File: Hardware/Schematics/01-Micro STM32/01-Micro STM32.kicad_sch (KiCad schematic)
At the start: 0 parts

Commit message: update
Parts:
- added J1: Screw_Terminal_01x04, symbol Connector:Screw_Terminal_01x04
- added U1: MCP23017_ML, Package_DFN_QFN:QFN-28-1EP_6x6mm_P0.65mm_EP4.25x4.25mm, symbol Interface_Expansion:MCP23017_ML
- added U2: ESP32-DEVKITC-32D, ESP32-DEVKITC-32D:MODULE_ESP32-DEVKITC-32D, symbol ESP32-DEVKITC-32D:ESP32-DEVKITC-32D
- added U3, U4: 74HCT138, symbol 74xx:74HCT138
- added U69A: AD8604ARUZ, AD8604ARUZ:SOP65P640X120-14N, symbol AD8604ARUZ:AD8604ARUZ

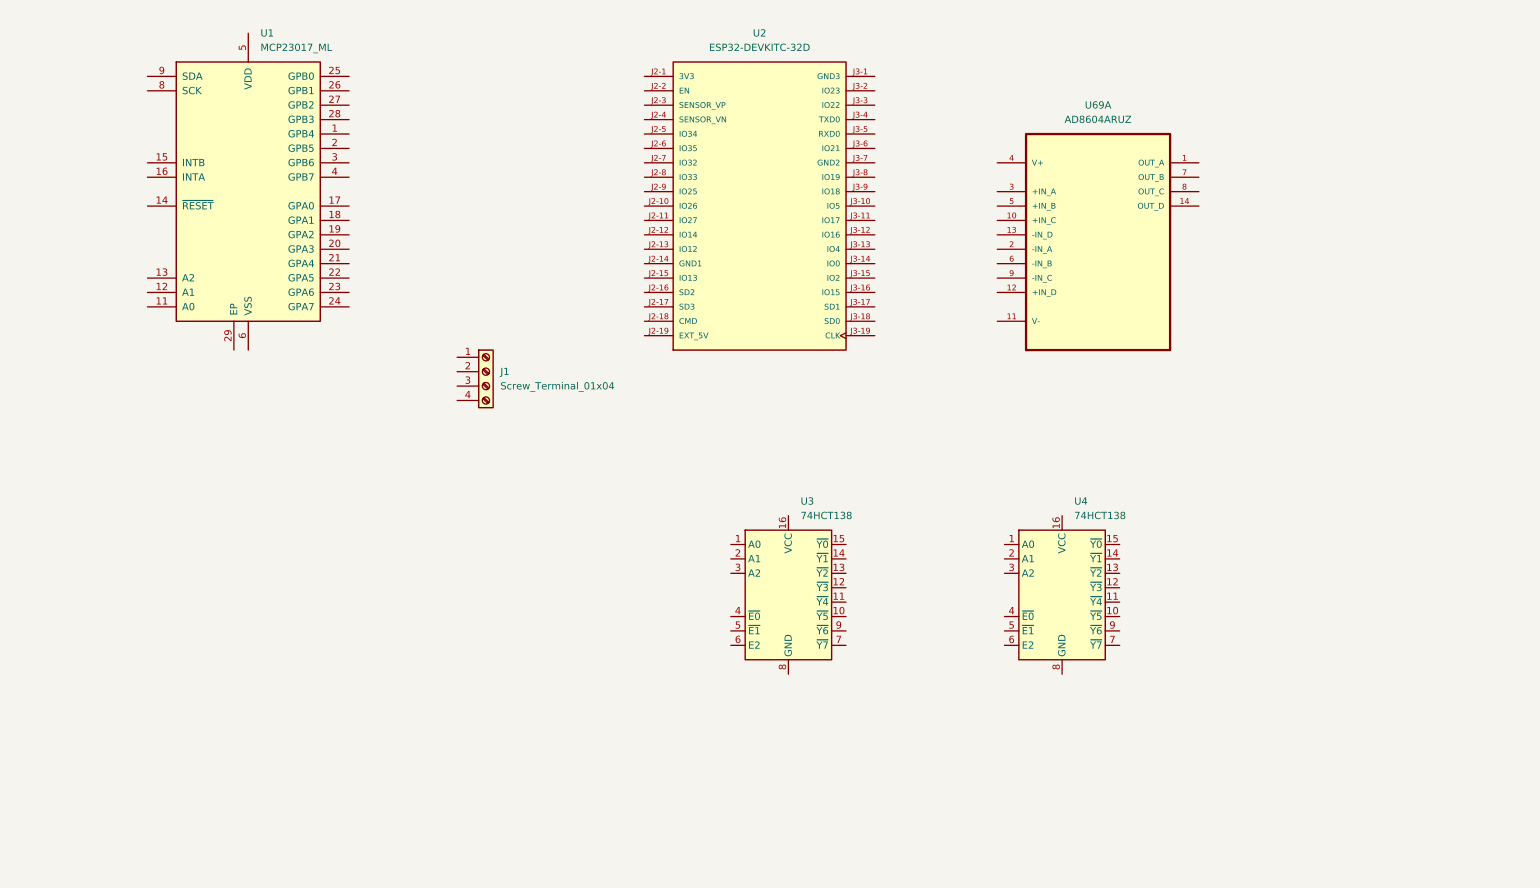
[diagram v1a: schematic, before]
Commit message: update
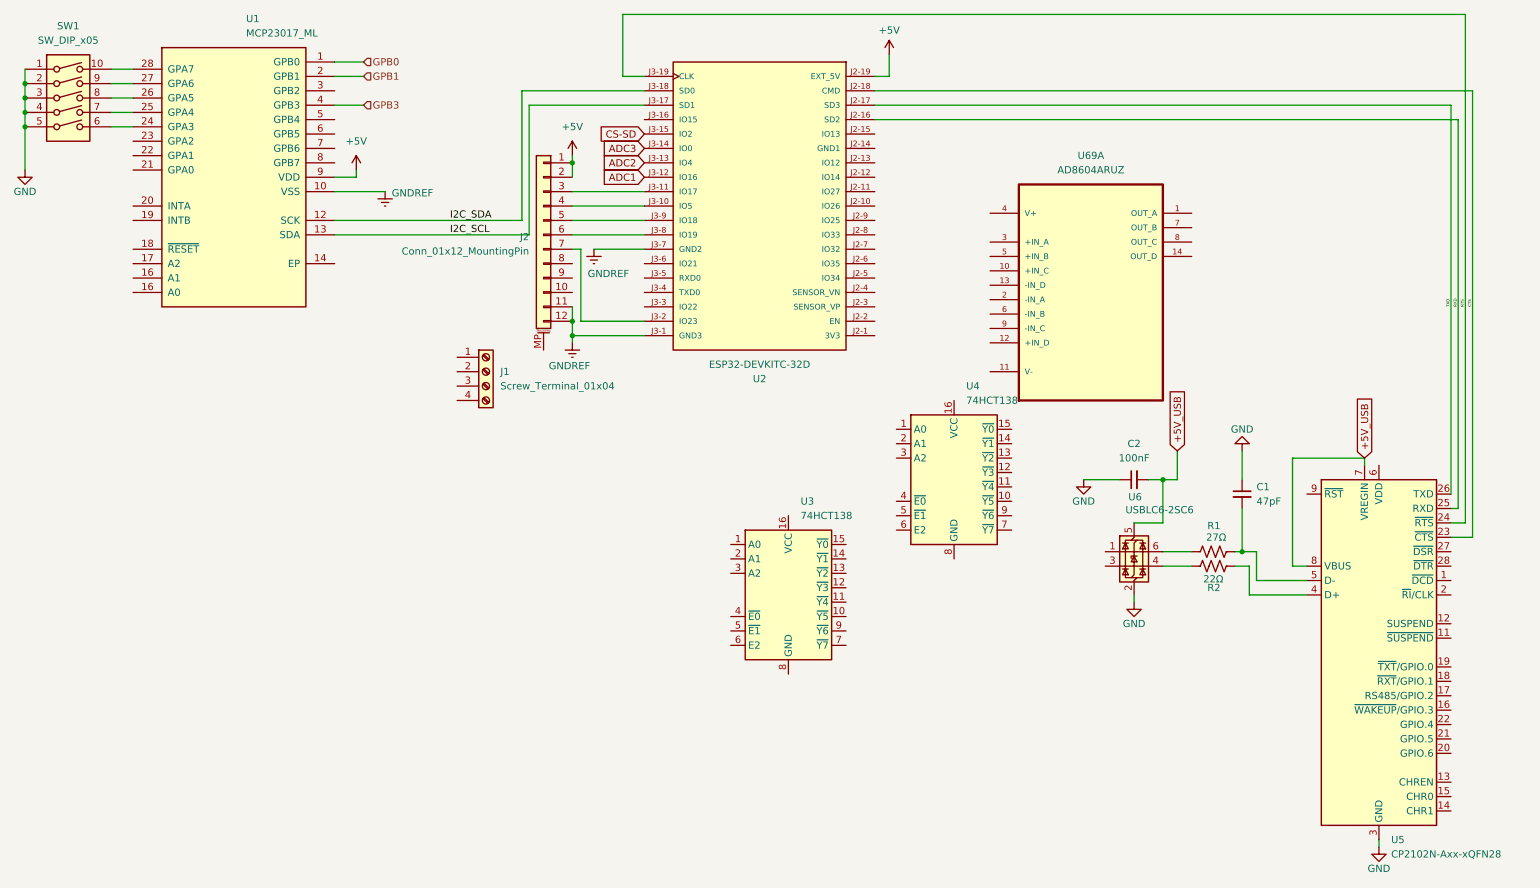
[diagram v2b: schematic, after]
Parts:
- added C1: 47pF, symbol Device:C_Small
- added C2: 100nF, symbol Device:C_Small
- added J2: Conn_01x12_MountingPin, symbol Connector_Generic_MountingPin:Conn_01x12_MountingPin
- added R1: 27Ω, symbol Device:R_US
- added R2: 22Ω, symbol Device:R_US
- added SW1: SW_DIP_x05, symbol Switch:SW_DIP_x05
- added U5: CP2102N-Axx-xQFN28, Package_DFN_QFN:QFN-28-1EP_5x5mm_P0.5mm_EP3.35x3.35mm, symbol Interface_USB:CP2102N-Axx-xQFN28
- added U6: USBLC6-2SC6, Package_TO_SOT_SMD:SOT-23-6, symbol Power_Protection:USBLC6-2SC6
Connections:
- net RXD: now reaches U2.J2-16 (SD2)
- net RXD: now also U5.25 (RXD)
- net TXD: now reaches U2.J2-17 (SD3)
- net TXD: now also U5.26 (TXD)
- net CTS: now reaches U2.J2-18 (CMD)
- net CTS: now also U5.23 (~{CTS})
- net +5V: now reaches U2.J2-19 (EXT_5V)
- net +5V: now also U1.9 (VDD), J2.1 (Pin_1), J2.2 (Pin_2)
- net GNDREF: now reaches U2.J3-1 (GND3)
- net GNDREF: now also U1.10 (VSS), U2.J3-7 (GND2), J2.11 (Pin_11), J2.12 (Pin_12)
- net at U2.J3-10 (IO5): now also J2.4 (Pin_4)
- net at U2.J3-11 (IO17): now also J2.3 (Pin_3)
- net ADC1: now reaches U2.J3-12 (IO16)
- net ADC2: now reaches U2.J3-13 (IO4)
- net ADC3: now reaches U2.J3-14 (IO0)
- net CS-SD: now reaches U2.J3-15 (IO2)
- net I2C_SCL: now reaches U2.J3-17 (SD1)
- net I2C_SCL: now also U1.13 (SDA)
- net I2C_SDA: now reaches U2.J3-18 (SD0)
- net I2C_SDA: now also U1.12 (SCK)
- net RTS: now reaches U2.J3-19 (CLK)
- net RTS: now also U5.24 (~{RTS})
- net at U2.J3-2 (IO23): now also J2.7 (Pin_7)
- net at U2.J3-8 (IO19): now also J2.6 (Pin_6)
- net at U2.J3-9 (IO18): now also J2.5 (Pin_5)
- net GPB0: now reaches U1.1 (GPB0)
- net GPB1: now reaches U1.2 (GPB1)
- net at U1.24 (GPA3): now also SW1.6
- net at U1.25 (GPA4): now also SW1.7
- net at U1.26 (GPA5): now also SW1.8
- net at U1.27 (GPA6): now also SW1.9
- net at U1.28 (GPA7): now also SW1.10
- net GPB3: now reaches U1.4 (GPB3)
- new net: R2.1, U6.4 (I/O2)
- new net: R2.2, U5.4 (D+)
- new net: R1.1, U6.6 (I/O1)
- new net: C1.2, R1.2, U5.5 (D-)
- new net +5V_USB: C2.2, U5.7 (VREGIN), U5.8 (VBUS), U6.5 (VBUS)
- new net GND: C1.1, C2.1, SW1.1, SW1.2, SW1.3, SW1.4, SW1.5, U5.29 (GND), U5.3 (GND), U6.2 (GND)
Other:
- moved on the sheet: U1, U2, U4, U69A
